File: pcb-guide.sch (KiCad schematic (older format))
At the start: 24 parts, among them SW1 SW_Push, U1 ATmega32U4-AU, Y1 16Mhz

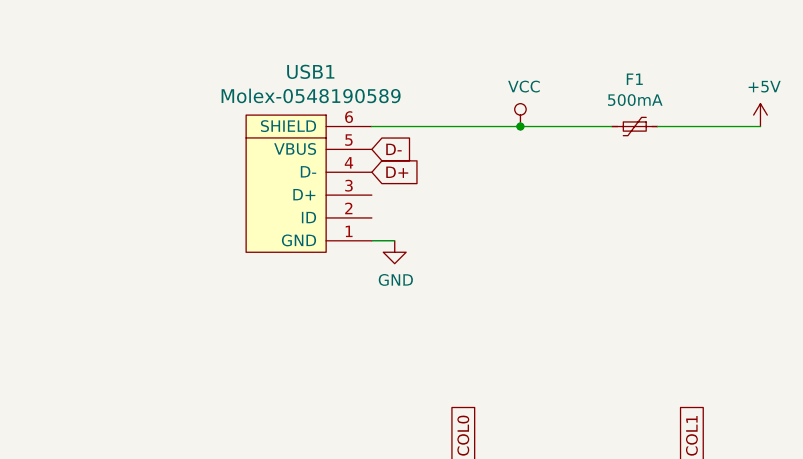
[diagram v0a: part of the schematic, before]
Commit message: PCB finished
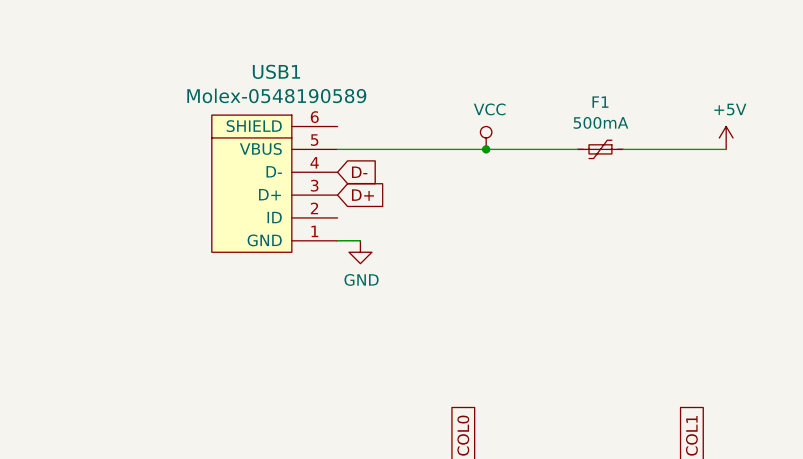
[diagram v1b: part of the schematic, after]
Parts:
- MX1, MX2, MX3, MX4: footprint MX_Alps_Hybrid:MX-1U -> MX_Only:MXOnly-1U
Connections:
- net D+: now also USB1.3 (D+); no longer USB1.4 (D-)
- net D-: now also USB1.4 (D-); no longer USB1.5 (VBUS)
- net VCC: now also USB1.5 (VBUS); no longer USB1.6 (SHIELD)
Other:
- moved on the sheet: F1, USB1
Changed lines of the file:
@@
 $EndComp
-Wire Wire Line
-	2950 4700 2850 4700
 Wire Wire Line
 	2850 4700 2450 4700
 Wire Wire Line
 	2450 4700 2450 4800
-Connection ~ 2850 4700
 $Comp
 L power:GND #PWR0103
@@
 L random-keyboard-parts:Molex-0548190589 USB1
 U 1 1 5FC20C0B
-P 5250 1550
-F 0 "USB1" V 5787 1517 60  0000 C CNN
-F 1 "Molex-0548190589" V 5681 1517 60  0000 C CNN
-F 2 "random-keyboard-parts:Molex-0548190589" H 5250 1550 60  0001 C CNN
-F 3 "" H 5250 1550 60  0001 C CNN
-	1    5250 1550
+P 5100 1550
+F 0 "USB1" V 5637 1517 60  0000 C CNN
+F 1 "Molex-0548190589" V 5531 1517 60  0000 C CNN
+F 2 "random-keyboard-parts:Molex-0548190589" H 5100 1550 60  0001 C CNN
+F 3 "" H 5100 1550 60  0001 C CNN
+	1    5100 1550
 	0    -1   -1   0
 $EndComp
-$Comp
-L power:VCC #PWR0110
-U 1 1 5FC21D9D
-P 6200 1250
-F 0 "#PWR0110" H 6200 1100 50  0001 C CNN
-F 1 "VCC" H 6217 1423 50  0000 C CNN
-F 2 "" H 6200 1250 50  0001 C CNN
-F 3 "" H 6200 1250 50  0001 C CNN
-	1    6200 1250
-	1    0    0    -1
-$EndComp
-$Comp
-L Device:Polyfuse_Small F1
-U 1 1 5FC22CD6
-P 6700 1250
-F 0 "F1" V 6495 1250 50  0000 C CNN
-F 1 "500mA" V 6586 1250 50  0000 C CNN
-F 2 "Fuse:Fuse_1206_3216Metric" H 6750 1050 50  0001 L CNN
-F 3 "~" H 6700 1250 50  0001 C CNN
-	1    6700 1250
-	0    1    1    0
-$EndComp
-$Comp
-L power:+5V #PWR0111
-U 1 1 5FC23944
-P 7250 1250
-F 0 "#PWR0111" H 7250 1100 50  0001 C CNN
-F 1 "+5V" H 7265 1423 50  0000 C CNN
-F 2 "" H 7250 1250 50  0001 C CNN
-F 3 "" H 7250 1250 50  0001 C CNN
-	1    7250 1250
-	1    0    0    -1
-$EndComp
-Wire Wire Line
-	5550 1250 6200 1250
-Wire Wire Line
-	6600 1250 6200 1250
-Connection ~ 6200 1250
-Wire Wire Line
-	6800 1250 7250 1250
-Text GLabel 5550 1450 2    50   Input ~ 0
+Text GLabel 5400 1550 2    50   Input ~ 0
 D+
-Text GLabel 5550 1350 2    50   Input ~ 0
+Text GLabel 5400 1450 2    50   Input ~ 0
 D-
 $Comp
 L power:GND #PWR0112
 U 1 1 5FC2A78A
-P 5650 1750
-F 0 "#PWR0112" H 5650 1500 50  0001 C CNN
-F 1 "GND" H 5655 1577 50  0000 C CNN
-F 2 "" H 5650 1750 50  0001 C CNN
-F 3 "" H 5650 1750 50  0001 C CNN
-	1    5650 1750
-	1    0    0    -1
-$EndComp
-Wire Wire Line
-	5550 1750 5650 1750
+P 5500 1750
+F 0 "#PWR0112" H 5500 1500 50  0001 C CNN
+F 1 "GND" H 5505 1577 50  0000 C CNN
+F 2 "" H 5500 1750 50  0001 C CNN
+F 3 "" H 5500 1750 50  0001 C CNN
+	1    5500 1750
+	1    0    0    -1
+$EndComp
+Wire Wire Line
+	5400 1750 5500 1750
 $Comp
 L MX_Alps_Hybrid:MX-NoLED MX1
@@
 F 0 "MX1" H 5833 3423 60  0000 C CNN
 F 1 "MX-NoLED" H 5833 3349 20  0000 C CNN
-F 2 "MX_Alps_Hybrid:MX-1U" H 5175 3175 60  0001 C CNN
+F 2 "MX_Only:MXOnly-1U" H 5175 3175 60  0001 C CNN
 F 3 "" H 5175 3175 60  0001 C CNN
 	1    5800 3200
@@
 F 0 "MX2" H 6833 3423 60  0000 C CNN
 F 1 "MX-NoLED" H 6833 3349 20  0000 C CNN
-F 2 "MX_Alps_Hybrid:MX-1U" H 6175 3175 60  0001 C CNN
+F 2 "MX_Only:MXOnly-1U" H 6175 3175 60  0001 C CNN
 F 3 "" H 6175 3175 60  0001 C CNN
 	1    6800 3200
@@
 F 0 "MX3" H 5833 4273 60  0000 C CNN
 F 1 "MX-NoLED" H 5833 4199 20  0000 C CNN
-F 2 "MX_Alps_Hybrid:MX-1U" H 5175 4025 60  0001 C CNN
+F 2 "MX_Only:MXOnly-1U" H 5175 4025 60  0001 C CNN
 F 3 "" H 5175 4025 60  0001 C CNN
 	1    5800 4050
@@
 F 0 "MX4" H 6833 4273 60  0000 C CNN
 F 1 "MX-NoLED" H 6833 4199 20  0000 C CNN
-F 2 "MX_Alps_Hybrid:MX-1U" H 6175 4025 60  0001 C CNN
+F 2 "MX_Only:MXOnly-1U" H 6175 4025 60  0001 C CNN
 F 3 "" H 6175 4025 60  0001 C CNN
 	1    6800 4050
@@
 Wire Wire Line
 	3950 3500 3550 3500
+Wire Wire Line
+	6650 1350 7100 1350
+Connection ~ 6050 1350
+Wire Wire Line
+	6450 1350 6050 1350
+Wire Wire Line
+	5400 1350 6050 1350
+$Comp
+L power:+5V #PWR0111
+U 1 1 5FC23944
+P 7100 1350
+F 0 "#PWR0111" H 7100 1200 50  0001 C CNN
+F 1 "+5V" H 7115 1523 50  0000 C CNN
+F 2 "" H 7100 1350 50  0001 C CNN
+F 3 "" H 7100 1350 50  0001 C CNN
+	1    7100 1350
+	1    0    0    -1
+$EndComp
+$Comp
+L Device:Polyfuse_Small F1
+U 1 1 5FC22CD6
+P 6550 1350
+F 0 "F1" V 6345 1350 50  0000 C CNN
+F 1 "500mA" V 6436 1350 50  0000 C CNN
+F 2 "Fuse:Fuse_1206_3216Metric" H 6600 1150 50  0001 L CNN
+F 3 "~" H 6550 1350 50  0001 C CNN
+	1    6550 1350
+	0    1    1    0
+$EndComp
+$Comp
+L power:VCC #PWR0110
+U 1 1 5FC21D9D
+P 6050 1350
+F 0 "#PWR0110" H 6050 1200 50  0001 C CNN
+F 1 "VCC" H 6067 1523 50  0000 C CNN
+F 2 "" H 6050 1350 50  0001 C CNN
+F 3 "" H 6050 1350 50  0001 C CNN
+	1    6050 1350
+	1    0    0    -1
+$EndComp
+Connection ~ 2850 4700
+Wire Wire Line
+	2950 4700 2850 4700
 $EndSCHEMATC
